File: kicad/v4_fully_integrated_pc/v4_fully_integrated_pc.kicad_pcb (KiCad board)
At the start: 2 copper layers, 25.7 x 39.9 mm, 21 parts, among them SW1 SW_Push, SW2 SW_Push, U1 nice_nano, U3 SSD1306_OLED_042, U4 SSD1306_OLED_042

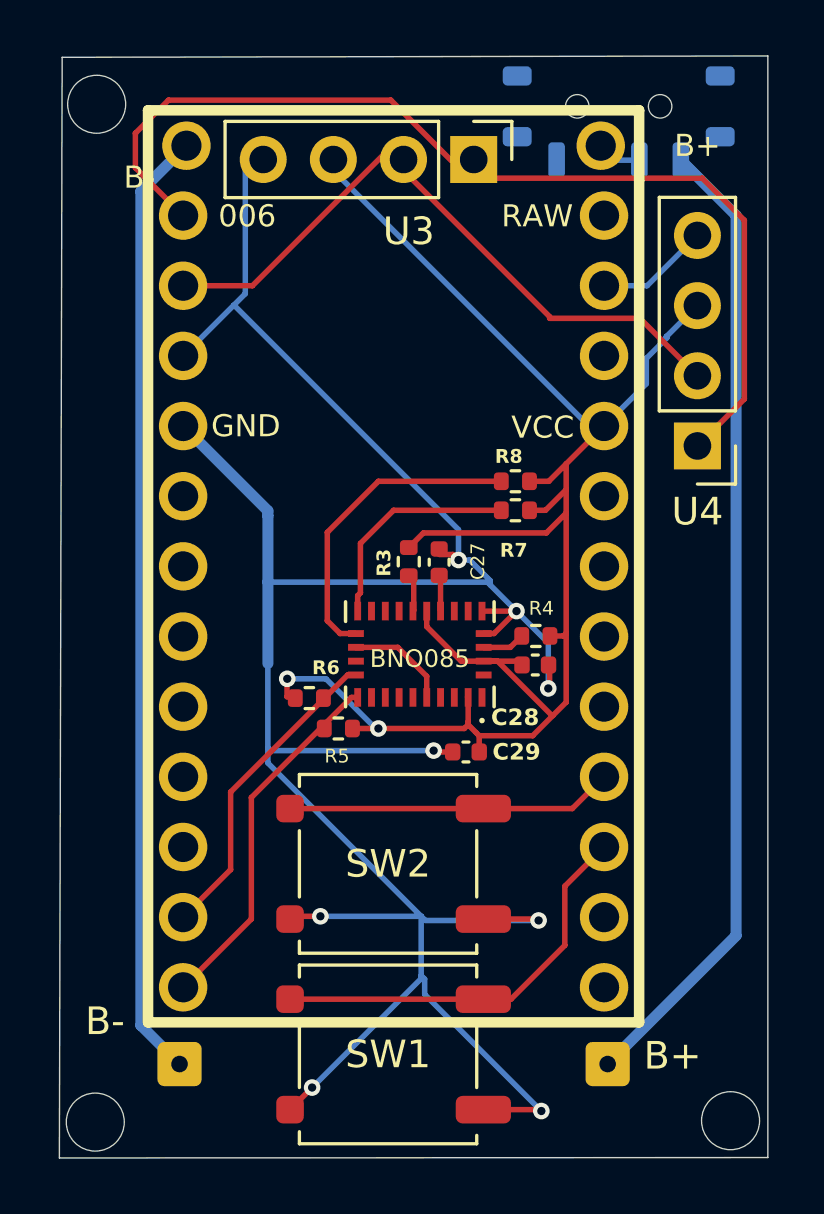
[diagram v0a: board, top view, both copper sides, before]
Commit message: before ref
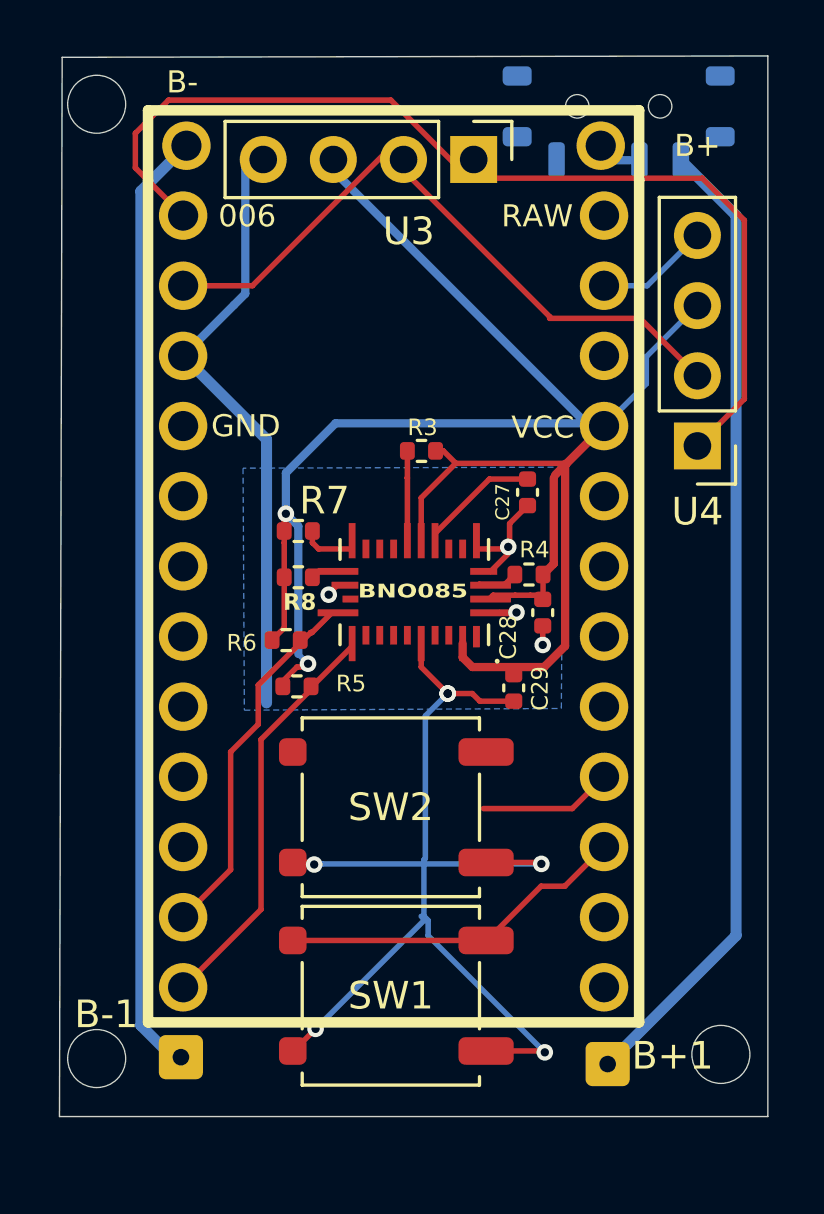
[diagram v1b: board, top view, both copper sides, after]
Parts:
- moved R8 8.59 mm to (174.3, 49.4), turned to 180 degrees
- moved R7 7.90 mm to (174.3, 47.7), turned to 180 degrees
- moved C27 4.08 mm to (182.6, 46.3), turned to 90 degrees
- moved R3 4.04 mm to (178.8, 44.8), turned to 0 degrees
- moved C29 2.89 mm to (182.1, 53.4), turned to 90 degrees
- moved REF** 2.43 mm to (189.6, 66.7)
- moved REF** 2.30 mm to (167.0, 66.8)
- moved R6 2.26 mm to (173.9, 51.6)
- moved BNO085 2.26 mm to (178.5, 49.9)
- moved R4 2.24 mm to (182.7, 49.3)
- moved R5 2.14 mm to (174.2, 53.3), turned to 180 degrees
- moved SW1 2.13 mm to (177.7, 64.5)
- moved SW2 2.05 mm to (177.7, 57.7)
- moved C28 1.91 mm to (183.2, 50.7), turned to 90 degrees
- moved B-1 0.25 mm to (170.1, 66.8)
- renumbered B+ to B+1, B- to B-1
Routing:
- net GND: track 104.8 -> 74.1 mm, vias 8 -> 10
- net PPH_VCC: track 64.0 -> 76.5 mm
- net Net-(BNO085-ENV_SDA): track 11.5 -> 1.47 mm
- net Net-(U1-P1.13): track 11.8 -> 4.85 mm
- net Net-(BNO085-ENV_SCL): track 8.09 -> 1.96 mm
- net Net-(BNO085-CAP): track 1.31 -> 4.73 mm
- net SCL_BNO: track 11.5 -> 14.0 mm
- net Net-(BNO085-~{RST}): track 1.16 -> 3.56 mm
- net Net-(U1-P1.11): track 14.9 -> 12.6 mm
- net SDA_BNO: track 13.2 -> 15.3 mm
- added copper zone on B.Cu, net GND
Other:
- board size 25.7 x 39.9 mm -> 25.6 x 38.4 mm
